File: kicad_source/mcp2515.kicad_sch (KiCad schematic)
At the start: 14 parts, among them CN4 GH_SM04B-GHS-TB, CN5 GH_SM04B-GHS-TB, U8 MCP2515, U9 SN65HVD232, Y1 16MHz

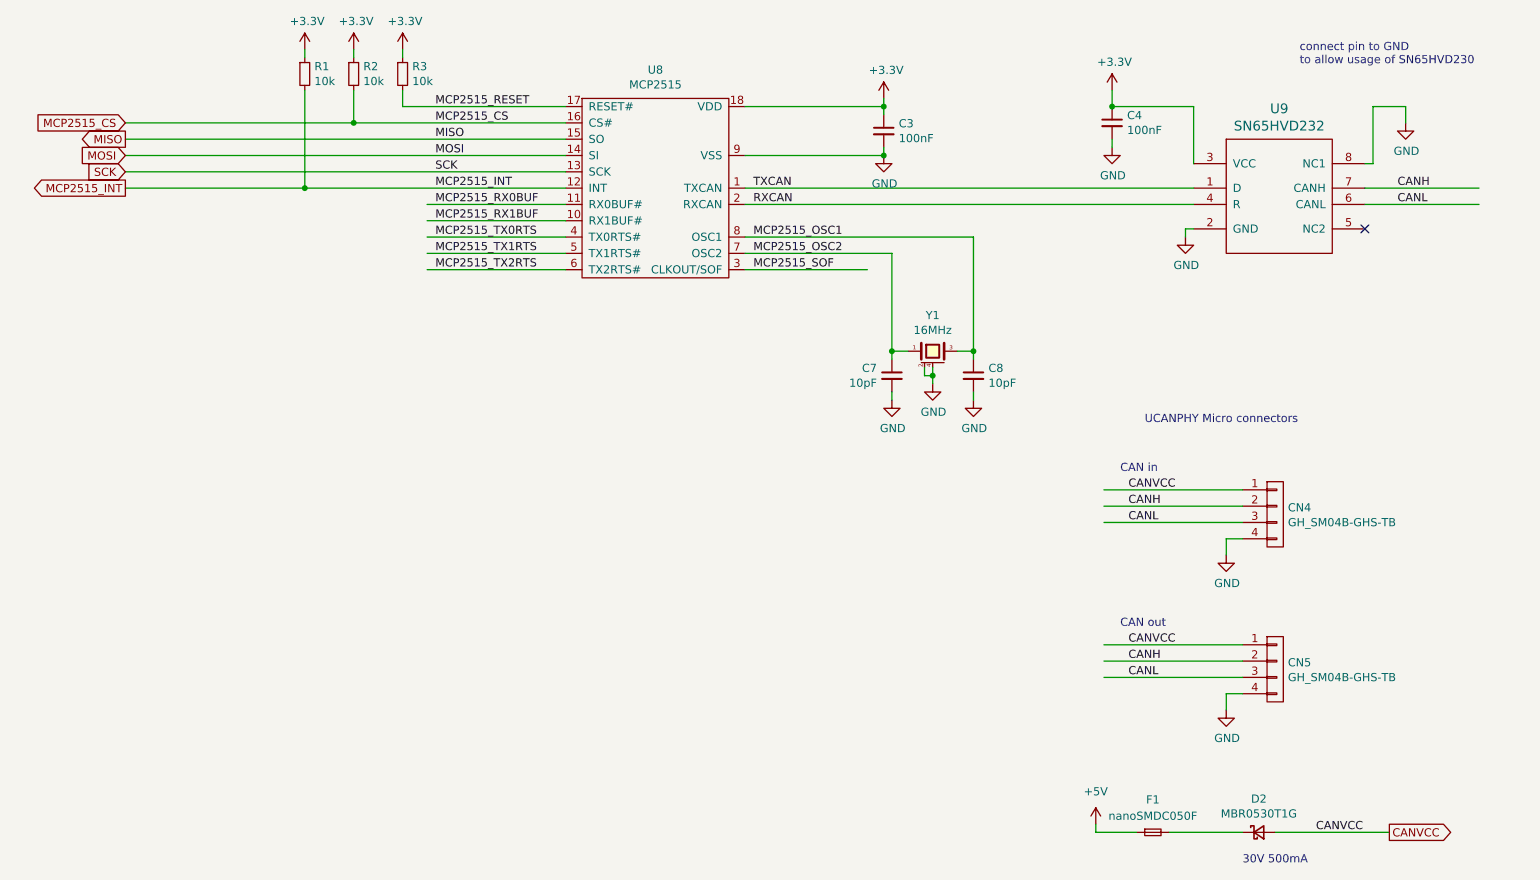
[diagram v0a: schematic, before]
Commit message: started first placement
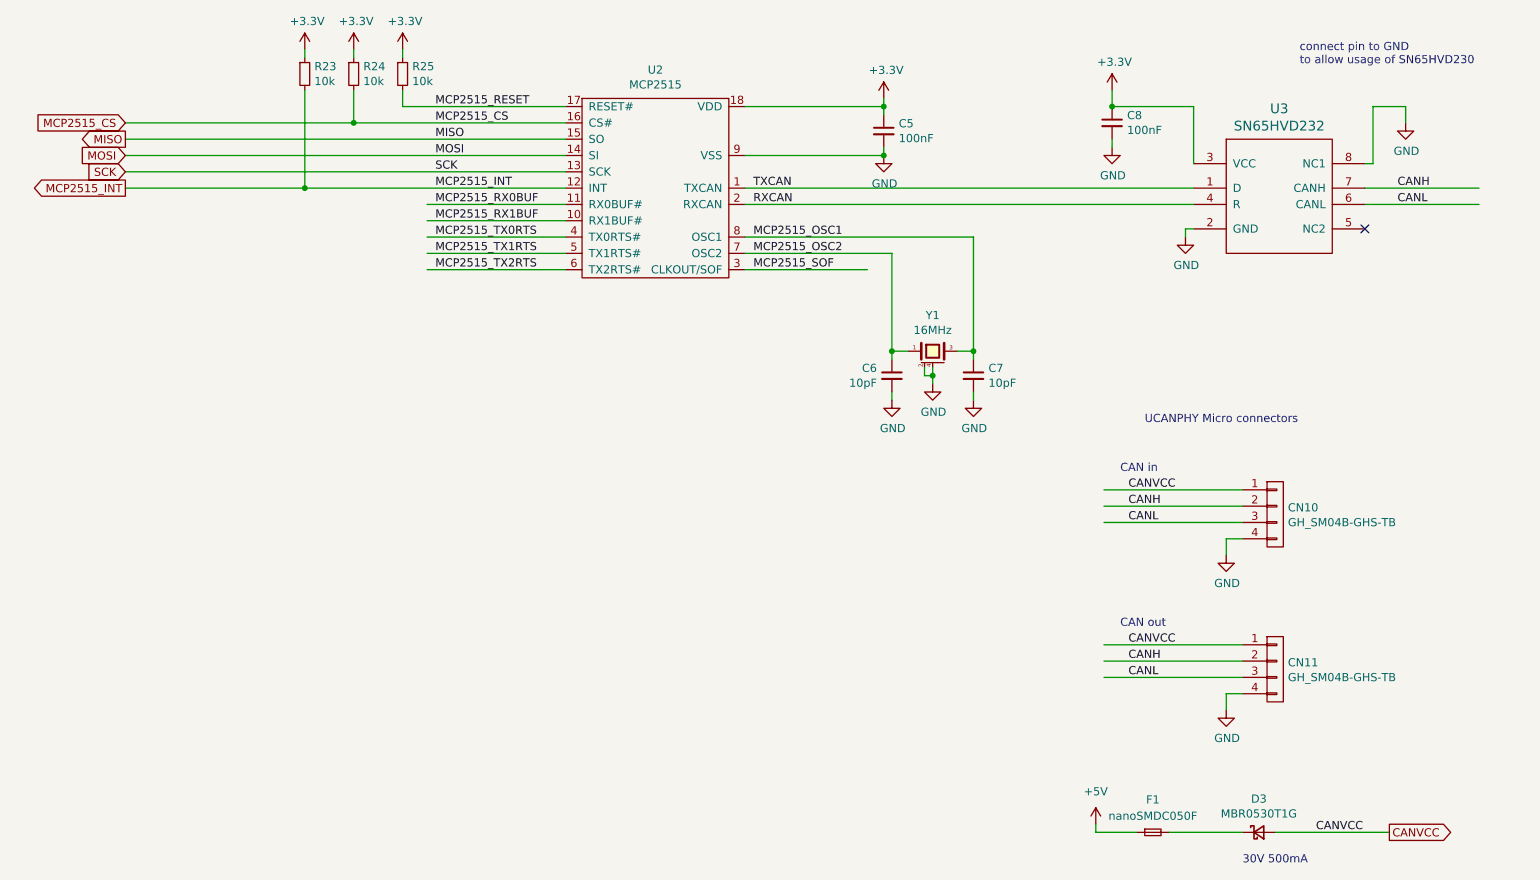
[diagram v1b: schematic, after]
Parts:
- renumbered C3 to C5, C7 to C6, C8 to C7, C4 to C8, CN4 to CN10, CN5 to CN11, D2 to D3, R1 to R23, R2 to R24, R3 to R25, U8 to U2, U9 to U3
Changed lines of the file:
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@@
   (symbol (lib_id "OpenCyphalPicoBase-rescue:MCP2515-IC_transceiver_can") (at 127 55.88 0) (unit 1)
     (in_bom yes) (on_board yes)
-    (property "Reference" "U8" (id 0) (at 127 37.465 0))
+    (property "Reference" "U2" (id 0) (at 127 37.465 0))
     (property "Value" "MCP2515" (id 1) (at 127 39.7764 0))
     (property "Footprint" "Package_SO:SOIC-18W_7.5x11.6mm_P1.27mm" (id 2) (at 127 55.88 0)
@@
   (symbol (lib_id "Device:C_Small") (at 162.56 46.99 0) (unit 1)
     (in_bom yes) (on_board yes)
-    (property "Reference" "C3" (id 0) (at 164.8968 45.8216 0)
+    (property "Reference" "C5" (id 0) (at 164.8968 45.8216 0)
       (effects (font (size 1.27 1.27)) (justify left))
     )
@@
   (symbol (lib_id "OpenCyphalPicoBase-rescue:+3.3V-power-supply") (at 162.56 41.91 0) (unit 1)
     (in_bom yes) (on_board yes)
-    (property "Reference" "#PWR025" (id 0) (at 162.56 45.72 0)
+    (property "Reference" "#PWR052" (id 0) (at 162.56 45.72 0)
       (effects (font (size 1.27 1.27)) hide)
     )
@@
   (symbol (lib_id "OpenCyphalPicoBase-rescue:GND-power-supply") (at 162.56 50.8 0) (unit 1)
     (in_bom yes) (on_board yes)
-    (property "Reference" "#PWR026" (id 0) (at 162.56 57.15 0)
+    (property "Reference" "#PWR053" (id 0) (at 162.56 57.15 0)
       (effects (font (size 1.27 1.27)) hide)
     )
@@
   (symbol (lib_id "OpenCyphalPicoBase-rescue:GND-power-supply") (at 170.18 86.36 0) (unit 1)
     (in_bom yes) (on_board yes)
-    (property "Reference" "#PWR027" (id 0) (at 170.18 92.71 0)
+    (property "Reference" "#PWR055" (id 0) (at 170.18 92.71 0)
       (effects (font (size 1.27 1.27)) hide)
     )
@@
   (symbol (lib_id "Device:R_Small") (at 87.63 38.1 0) (unit 1)
     (in_bom yes) (on_board yes)
-    (property "Reference" "R3" (id 0) (at 89.1286 36.9316 0)
+    (property "Reference" "R25" (id 0) (at 89.1286 36.9316 0)
       (effects (font (size 1.27 1.27)) (justify left))
     )
@@
   (symbol (lib_id "OpenCyphalPicoBase-rescue:+3.3V-power-supply") (at 87.63 34.29 0) (unit 1)
     (in_bom yes) (on_board yes)
-    (property "Reference" "#PWR024" (id 0) (at 87.63 38.1 0)
+    (property "Reference" "#PWR051" (id 0) (at 87.63 38.1 0)
       (effects (font (size 1.27 1.27)) hide)
     )
@@
   (symbol (lib_id "Device:R_Small") (at 80.01 38.1 0) (unit 1)
     (in_bom yes) (on_board yes)
-    (property "Reference" "R2" (id 0) (at 81.5086 36.9316 0)
+    (property "Reference" "R24" (id 0) (at 81.5086 36.9316 0)
       (effects (font (size 1.27 1.27)) (justify left))
     )
@@
   (symbol (lib_id "OpenCyphalPicoBase-rescue:+3.3V-power-supply") (at 80.01 34.29 0) (unit 1)
     (in_bom yes) (on_board yes)
-    (property "Reference" "#PWR023" (id 0) (at 80.01 38.1 0)
+    (property "Reference" "#PWR050" (id 0) (at 80.01 38.1 0)
       (effects (font (size 1.27 1.27)) hide)
     )
@@
   (symbol (lib_id "Device:R_Small") (at 72.39 38.1 0) (unit 1)
     (in_bom yes) (on_board yes)
-    (property "Reference" "R1" (id 0) (at 73.8886 36.9316 0)
+    (property "Reference" "R23" (id 0) (at 73.8886 36.9316 0)
       (effects (font (size 1.27 1.27)) (justify left))
     )
@@
   (symbol (lib_id "OpenCyphalPicoBase-rescue:+3.3V-power-supply") (at 72.39 34.29 0) (unit 1)
     (in_bom yes) (on_board yes)
-    (property "Reference" "#PWR022" (id 0) (at 72.39 38.1 0)
+    (property "Reference" "#PWR049" (id 0) (at 72.39 38.1 0)
       (effects (font (size 1.27 1.27)) hide)
     )
@@
   (symbol (lib_id "OpenCyphalPicoBase-rescue:SN65HVD232-CAN-transceiver") (at 210.82 66.04 0) (unit 1)
     (in_bom yes) (on_board yes)
-    (property "Reference" "U9" (id 0) (at 224.155 43.5102 0)
+    (property "Reference" "U3" (id 0) (at 224.155 43.5102 0)
       (effects (font (size 1.524 1.524)))
     )
@@
   (symbol (lib_id "Device:C_Small") (at 198.12 45.72 0) (unit 1)
     (in_bom yes) (on_board yes)
-    (property "Reference" "C4" (id 0) (at 200.4568 44.5516 0)
+    (property "Reference" "C8" (id 0) (at 200.4568 44.5516 0)
       (effects (font (size 1.27 1.27)) (justify left))
     )
@@
   (symbol (lib_id "OpenCyphalPicoBase-rescue:+3.3V-power-supply") (at 198.12 40.64 0) (unit 1)
     (in_bom yes) (on_board yes)
-    (property "Reference" "#PWR028" (id 0) (at 198.12 44.45 0)
+    (property "Reference" "#PWR058" (id 0) (at 198.12 44.45 0)
       (effects (font (size 1.27 1.27)) hide)
     )
@@
   (symbol (lib_id "OpenCyphalPicoBase-rescue:GND-power-supply") (at 198.12 49.53 0) (unit 1)
     (in_bom yes) (on_board yes)
-    (property "Reference" "#PWR029" (id 0) (at 198.12 55.88 0)
+    (property "Reference" "#PWR059" (id 0) (at 198.12 55.88 0)
       (effects (font (size 1.27 1.27)) hide)
     )
@@
   (symbol (lib_id "OpenCyphalPicoBase-rescue:GND-power-supply") (at 209.55 63.5 0) (unit 1)
     (in_bom yes) (on_board yes)
-    (property "Reference" "#PWR030" (id 0) (at 209.55 69.85 0)
+    (property "Reference" "#PWR060" (id 0) (at 209.55 69.85 0)
       (effects (font (size 1.27 1.27)) hide)
     )
@@
   (symbol (lib_id "OpenCyphalPicoBase-rescue:CONN_01X04-mechanical-connectors") (at 223.52 106.68 0) (unit 1)
     (in_bom yes) (on_board yes)
-    (property "Reference" "CN4" (id 0) (at 225.5012 105.6386 0)
+    (property "Reference" "CN10" (id 0) (at 225.5012 105.6386 0)
       (effects (font (size 1.27 1.27)) (justify left))
     )
@@
   (symbol (lib_id "OpenCyphalPicoBase-rescue:GND-power-supply") (at 215.9 113.03 0) (unit 1)
     (in_bom yes) (on_board yes)
-    (property "Reference" "#PWR036" (id 0) (at 215.9 119.38 0)
+    (property "Reference" "#PWR061" (id 0) (at 215.9 119.38 0)
       (effects (font (size 1.27 1.27)) hide)
     )
@@
   (symbol (lib_id "OpenCyphalPicoBase-rescue:CONN_01X04-mechanical-connectors") (at 223.52 130.81 0) (unit 1)
     (in_bom yes) (on_board yes)
-    (property "Reference" "CN5" (id 0) (at 225.5012 129.7686 0)
+    (property "Reference" "CN11" (id 0) (at 225.5012 129.7686 0)
       (effects (font (size 1.27 1.27)) (justify left))
     )
@@
   (symbol (lib_id "OpenCyphalPicoBase-rescue:GND-power-supply") (at 215.9 137.16 0) (unit 1)
     (in_bom yes) (on_board yes)
-    (property "Reference" "#PWR037" (id 0) (at 215.9 143.51 0)
+    (property "Reference" "#PWR062" (id 0) (at 215.9 143.51 0)
       (effects (font (size 1.27 1.27)) hide)
     )
@@
   (symbol (lib_id "Device:D_Schottky_Small") (at 220.98 156.21 0) (unit 1)
     (in_bom yes) (on_board yes)
-    (property "Reference" "D2" (id 0) (at 220.98 151.003 0))
+    (property "Reference" "D3" (id 0) (at 220.98 151.003 0))
     (property "Value" "MBR0530T1G" (id 1) (at 220.98 153.3144 0))
     (property "Footprint" "Diode_SMD:D_SOD-123" (id 2) (at 220.98 156.21 90)
@@
   (symbol (lib_id "Device:C_Small") (at 176.53 85.09 0) (unit 1)
     (in_bom yes) (on_board yes)
-    (property "Reference" "C8" (id 0) (at 178.8668 83.9216 0)
+    (property "Reference" "C7" (id 0) (at 178.8668 83.9216 0)
       (effects (font (size 1.27 1.27)) (justify left))
     )
@@
   (symbol (lib_id "Device:C_Small") (at 163.83 85.09 0) (mirror y) (unit 1)
     (in_bom yes) (on_board yes)
-    (property "Reference" "C7" (id 0) (at 161.4932 83.9216 0)
+    (property "Reference" "C6" (id 0) (at 161.4932 83.9216 0)
       (effects (font (size 1.27 1.27)) (justify left))
     )
@@
   (symbol (lib_id "OpenCyphalPicoBase-rescue:GND-power-supply") (at 163.83 88.9 0) (unit 1)
     (in_bom yes) (on_board yes)
-    (property "Reference" "#PWR034" (id 0) (at 163.83 95.25 0)
+    (property "Reference" "#PWR054" (id 0) (at 163.83 95.25 0)
       (effects (font (size 1.27 1.27)) hide)
     )
@@
   (symbol (lib_id "OpenCyphalPicoBase-rescue:GND-power-supply") (at 176.53 88.9 0) (unit 1)
     (in_bom yes) (on_board yes)
-    (property "Reference" "#PWR035" (id 0) (at 176.53 95.25 0)
+    (property "Reference" "#PWR056" (id 0) (at 176.53 95.25 0)
       (effects (font (size 1.27 1.27)) hide)
     )
@@
   (symbol (lib_id "OpenCyphalPicoBase-rescue:GND-power-supply") (at 243.84 45.72 0) (unit 1)
     (in_bom yes) (on_board yes)
-    (property "Reference" "#PWR0102" (id 0) (at 243.84 52.07 0)
+    (property "Reference" "#PWR063" (id 0) (at 243.84 52.07 0)
       (effects (font (size 1.27 1.27)) hide)
     )
@@
   (symbol (lib_id "power:+5V") (at 195.58 154.94 0) (unit 1)
     (in_bom yes) (on_board yes) (fields_autoplaced)
-    (property "Reference" "#PWR?" (id 0) (at 195.58 158.75 0)
-      (effects (font (size 1.27 1.27)) hide)
-    )
+    (property "Reference" "#PWR057" (id 0) (at 195.58 158.75 0)
+      (effects (font (size 1.27 1.27)) hide)
+    )
